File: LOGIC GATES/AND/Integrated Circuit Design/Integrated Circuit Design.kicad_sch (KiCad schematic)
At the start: 13 parts, among them J1 Conn_01x03_Socket, J2 Conn_01x03_Socket, J3 Conn_01x03_Socket, Q1 QM6006D, Q2 QM6006D, Q3 QM6006D, U1 4011

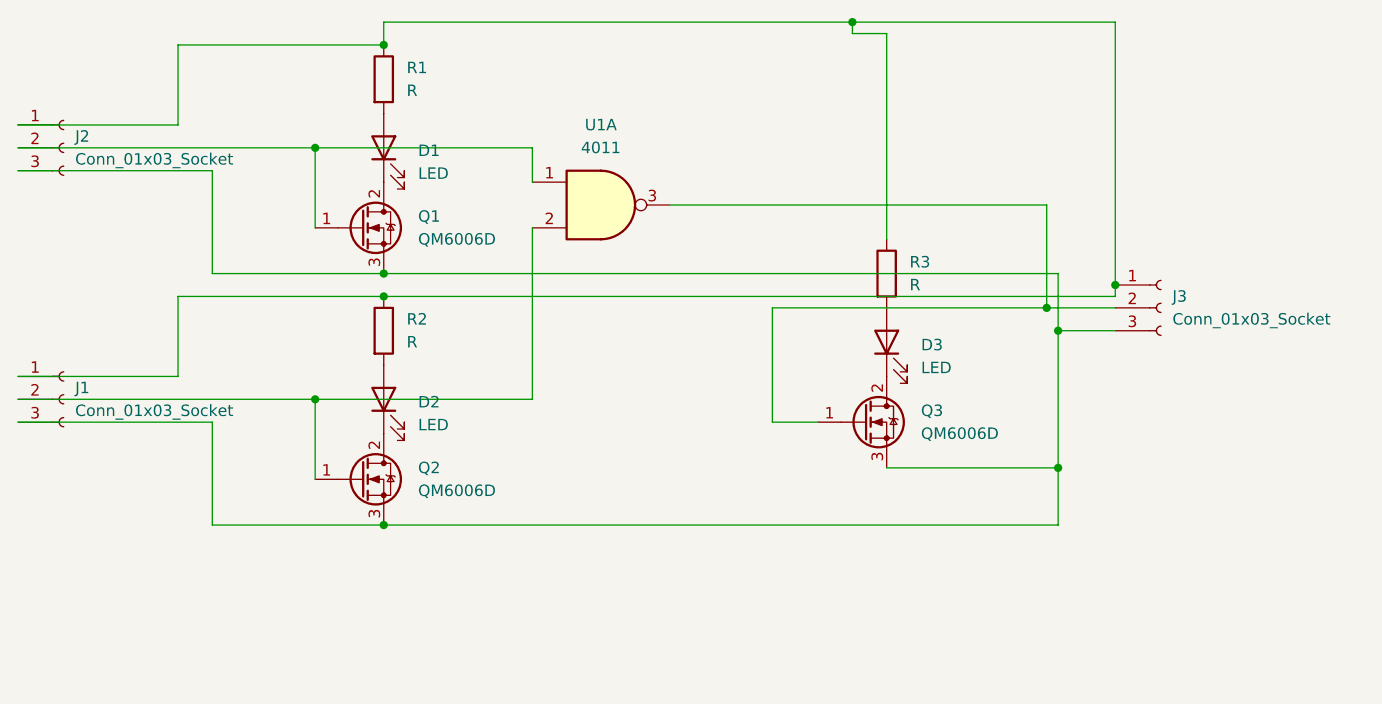
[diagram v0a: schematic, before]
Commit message: Auto-update: 21.12.2025 12:47:00,10
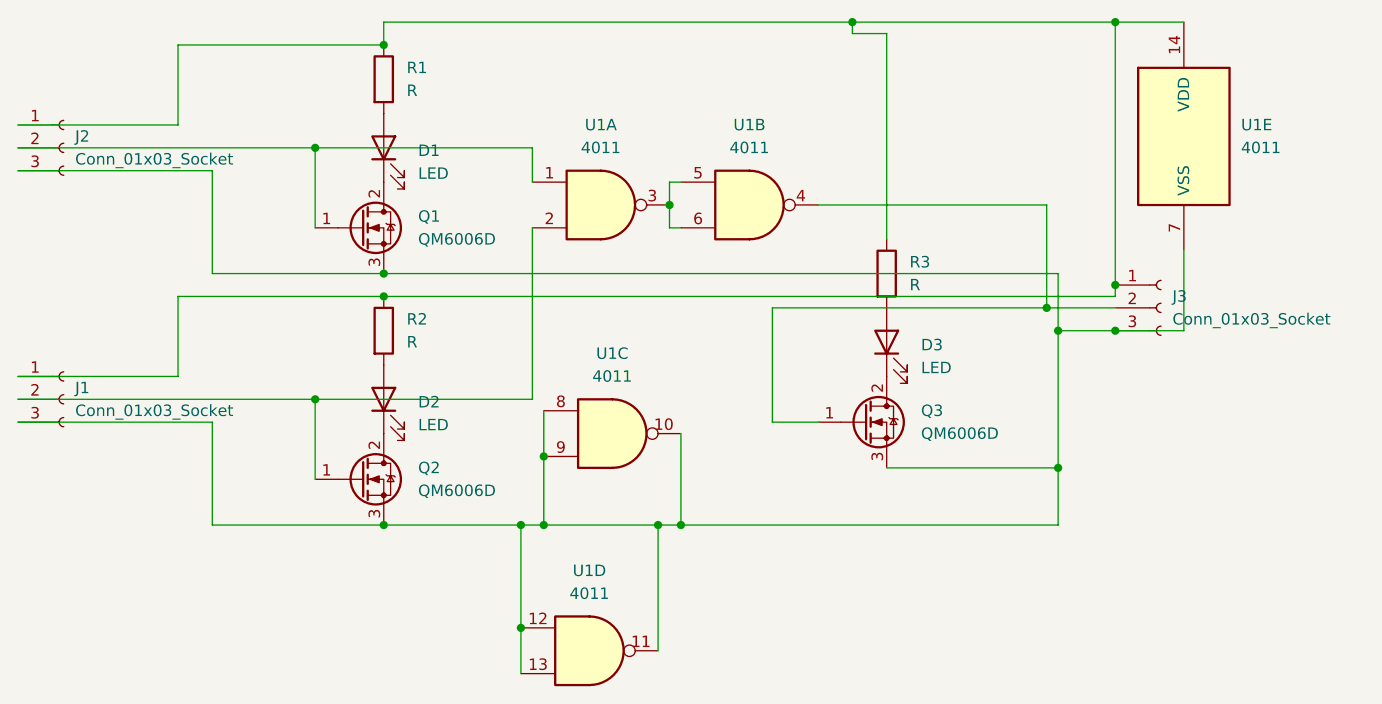
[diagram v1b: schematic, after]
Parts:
- added unit 3 of U1
- added unit 2 of U1
- added unit 4 of U1
- added unit 5 of U1
- U1: footprint (none) -> Package_DIP:DIP-14_W7.62mm_Socket
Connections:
- net at J3.2 (Pin_2), Q3.1 (G): now also U1.4; no longer U1.3
- net at J1.1 (Pin_1), J2.1 (Pin_1), J3.1 (Pin_1)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: now also U1.14 (VDD)
- net at J1.3 (Pin_3), J2.3 (Pin_3), J3.3 (Pin_3)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: now also U1.10, U1.11, U1.12, U1.13, U1.7 (VSS), U1.8, U1.9
- new net: U1.3, U1.5, U1.6

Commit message: Auto-update: 21.12.2025 13:35:58,67
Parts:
- U1: footprint Package_DIP:DIP-14_W7.62mm_Socket -> Package_DIP:DIP-14_W7.62mm
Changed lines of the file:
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@@
 			)
 		)
-		(property "Footprint" "Package_DIP:DIP-14_W7.62mm_Socket"
+		(property "Footprint" "Package_DIP:DIP-14_W7.62mm"
 			(at 82.55 78.74 0)
 			(effects
@@
 			)
 		)
-		(property "Footprint" "Package_DIP:DIP-14_W7.62mm_Socket"
+		(property "Footprint" "Package_DIP:DIP-14_W7.62mm"
 			(at 83.82 104.14 0)
 			(effects
@@
 			)
 		)
-		(property "Footprint" "Package_DIP:DIP-14_W7.62mm_Socket"
+		(property "Footprint" "Package_DIP:DIP-14_W7.62mm"
 			(at 99.06 78.74 0)
 			(effects
@@
 			)
 		)
-		(property "Footprint" "Package_DIP:DIP-14_W7.62mm_Socket"
+		(property "Footprint" "Package_DIP:DIP-14_W7.62mm"
 			(at 81.28 128.27 0)
 			(effects
@@
 			)
 		)
-		(property "Footprint" "Package_DIP:DIP-14_W7.62mm_Socket"
+		(property "Footprint" "Package_DIP:DIP-14_W7.62mm"
 			(at 147.32 71.12 0)
 			(effects
